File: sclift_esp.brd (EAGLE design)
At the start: 50.5 x 44.4 mm, 18 parts

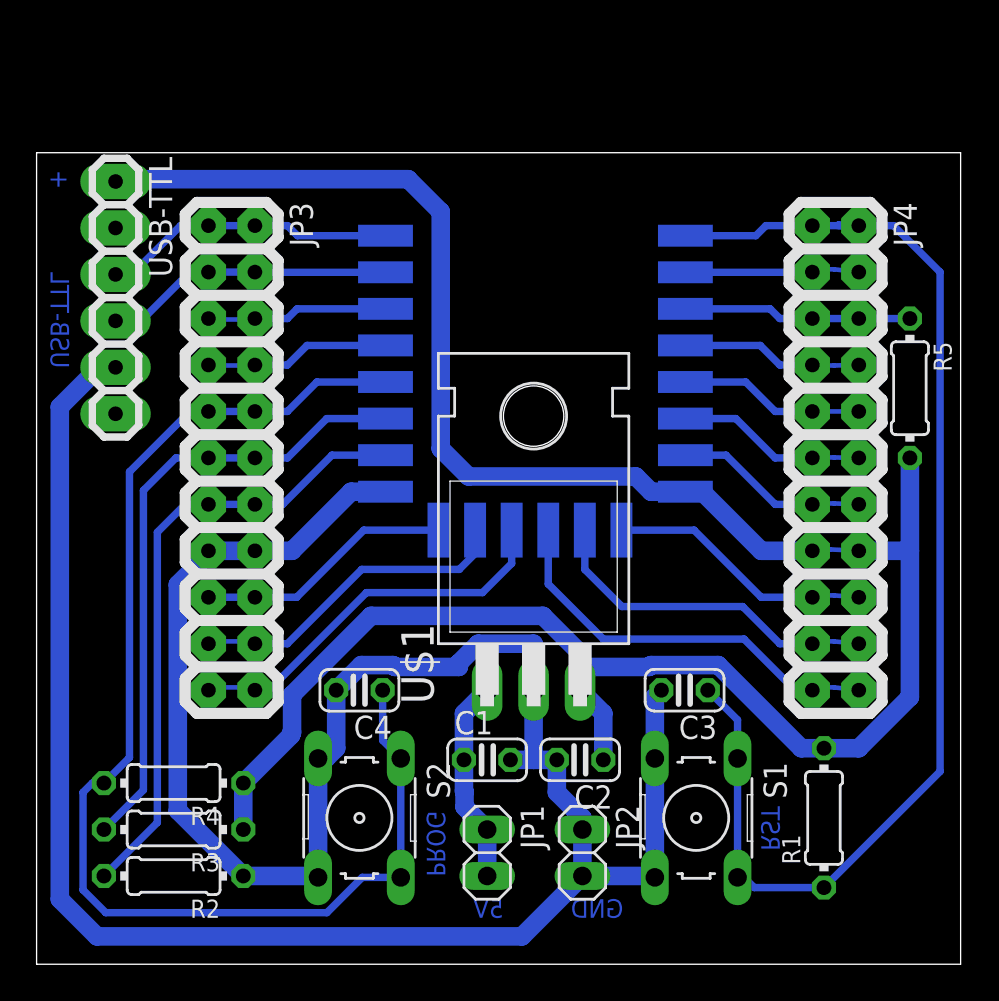
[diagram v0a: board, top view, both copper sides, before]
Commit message: Add files via upload
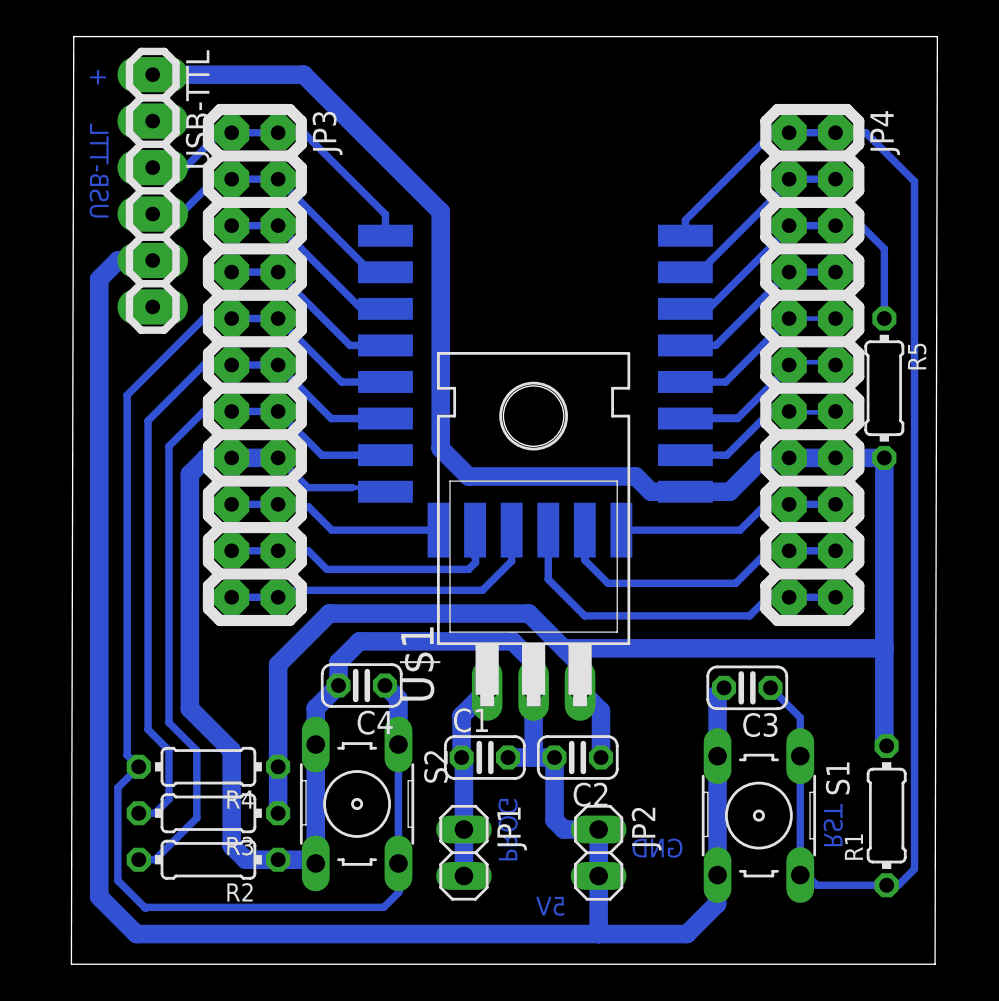
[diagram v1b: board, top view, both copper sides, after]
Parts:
- moved USB-TTL 6.19 mm to (6.35, 42.3)
- moved JP4 5.24 mm to (42.4, 32.8)
- moved JP3 5.24 mm to (11.9, 32.8)
- moved C3 3.43 mm to (38.9, 15.1)
- moved R1 3.43 mm to (46.5, 8.13)
- moved S1 3.43 mm to (39.5, 8.13)
- moved R3 2.10 mm to (9.40, 8.26)
- moved R2 2.10 mm to (9.40, 5.71)
- moved R4 2.10 mm to (9.40, 10.8)
- moved R5 1.40 mm to (46.4, 31.5)
- moved JP1 1.27 mm to (23.4, 6.10)
- moved JP2 0.89 mm to (30.7, 6.10)
- moved S2 0.77 mm to (17.5, 8.76)
- moved C4 0.28 mm to (17.8, 15.2)
- moved C1 0.18 mm to (24.5, 11.3)
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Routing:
- net GND: track 149.3 -> 165.3 mm
- net GPIO12: track 12.1 -> 16.9 mm
- net CHPD: track 12.5 -> 17.2 mm
- net CS0: track 16.7 -> 12.3 mm
- net MISO: track 21.0 -> 16.6 mm
- net GPIO2: track 34.3 -> 38.6 mm
- net GPIO15: track 34.4 -> 38.7 mm
- net 3V3: track 129.4 -> 125.2 mm
- net GPIO9: track 23.4 -> 19.8 mm
- net GPIO10: track 21.4 -> 17.8 mm
- net GPIO0: track 69.7 -> 73.1 mm
- net RESET: track 69.7 -> 72.1 mm
- net MOSI: track 18.0 -> 15.7 mm
- net SCLK: track 14.1 -> 11.9 mm
- net GPIO13: track 12.3 -> 10.2 mm
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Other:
- board size 50.5 x 44.4 mm -> 47.4 x 50.7 mm

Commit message: Add files via upload
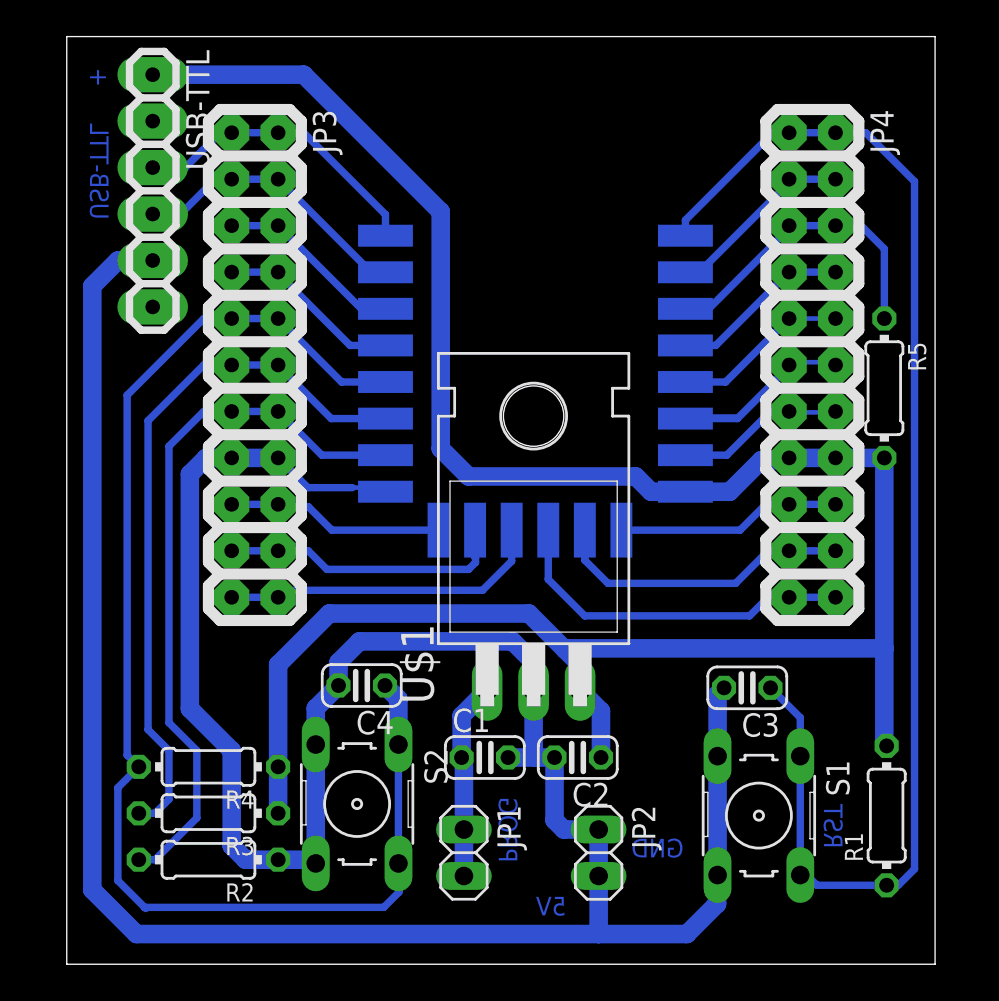
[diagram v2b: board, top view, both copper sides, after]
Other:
- board size 47.4 x 50.7 mm -> 47.5 x 50.7 mm
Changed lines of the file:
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@@
 <board>
 <plain>
-<wire x1="1.905" y1="0" x2="49.129" y2="0" width="0" layer="20"/>
-<wire x1="49.129" y1="0" x2="49.256" y2="50.724" width="0" layer="20"/>
-<wire x1="49.256" y1="50.724" x2="2.032" y2="50.724" width="0" layer="20"/>
-<wire x1="2.032" y1="50.724" x2="1.905" y2="0" width="0" layer="20"/>
+<wire x1="1.651" y1="0" x2="49.129" y2="0" width="0" layer="20"/>
+<wire x1="49.129" y1="0" x2="49.129" y2="50.724" width="0" layer="20"/>
+<wire x1="49.129" y1="50.724" x2="1.651" y2="50.724" width="0" layer="20"/>
+<wire x1="1.651" y1="50.724" x2="1.651" y2="0" width="0" layer="20"/>
 <text x="26.289" y="9.144" size="1.016" layer="16" rot="MR270">PROG</text>
 <text x="44.069" y="8.763" size="1.016" layer="16" rot="MR270">RST</text>
@@
 <wire x1="27.178" y1="16.51" x2="27.178" y2="14.986" width="1.016" layer="16"/>
 <wire x1="27.178" y1="16.51" x2="26.035" y2="17.653" width="1.016" layer="16"/>
-<wire x1="3.429" y1="37.465" x2="4.445" y2="38.481" width="1.016" layer="16"/>
 <wire x1="4.445" y1="38.481" x2="6.35" y2="38.481" width="1.016" layer="16"/>
-<wire x1="5.461" y1="1.651" x2="3.429" y2="3.683" width="1.016" layer="16"/>
 <wire x1="30.734" y1="1.651" x2="5.461" y2="1.651" width="1.016" layer="16"/>
-<wire x1="3.429" y1="3.683" x2="3.429" y2="37.465" width="1.016" layer="16"/>
 <wire x1="27.178" y1="14.986" x2="27.178" y2="11.43" width="1.016" layer="16"/>
 <wire x1="27.178" y1="11.43" x2="27.305" y2="11.303" width="1.016" layer="16"/>
@@
 <wire x1="17.272" y1="26.0604" x2="14.8336" y2="26.0604" width="0.4064" layer="16"/>
 <wire x1="14.8336" y1="26.0604" x2="13.208" y2="27.686" width="0.4064" layer="16"/>
+<wire x1="5.461" y1="1.651" x2="3.048" y2="4.064" width="1.016" layer="16"/>
+<wire x1="3.048" y1="37.084" x2="4.445" y2="38.481" width="1.016" layer="16"/>
+<wire x1="3.048" y1="4.064" x2="3.048" y2="37.084" width="1.016" layer="16"/>
 </signal>
 <signal name="RX">
